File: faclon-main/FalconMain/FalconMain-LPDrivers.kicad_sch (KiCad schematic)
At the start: 41 parts, among them Q17 Q_NMOS_GSD, Q18 Q_NMOS_GSD, Q19 Q_PMOS_LFPAK, Q20 Q_NMOS_GSD, Q21 Q_PMOS_GSD, U4 BD9E104FJ-E2, U5 AL8843QSP-13, U6 NCP164ASN330T1G

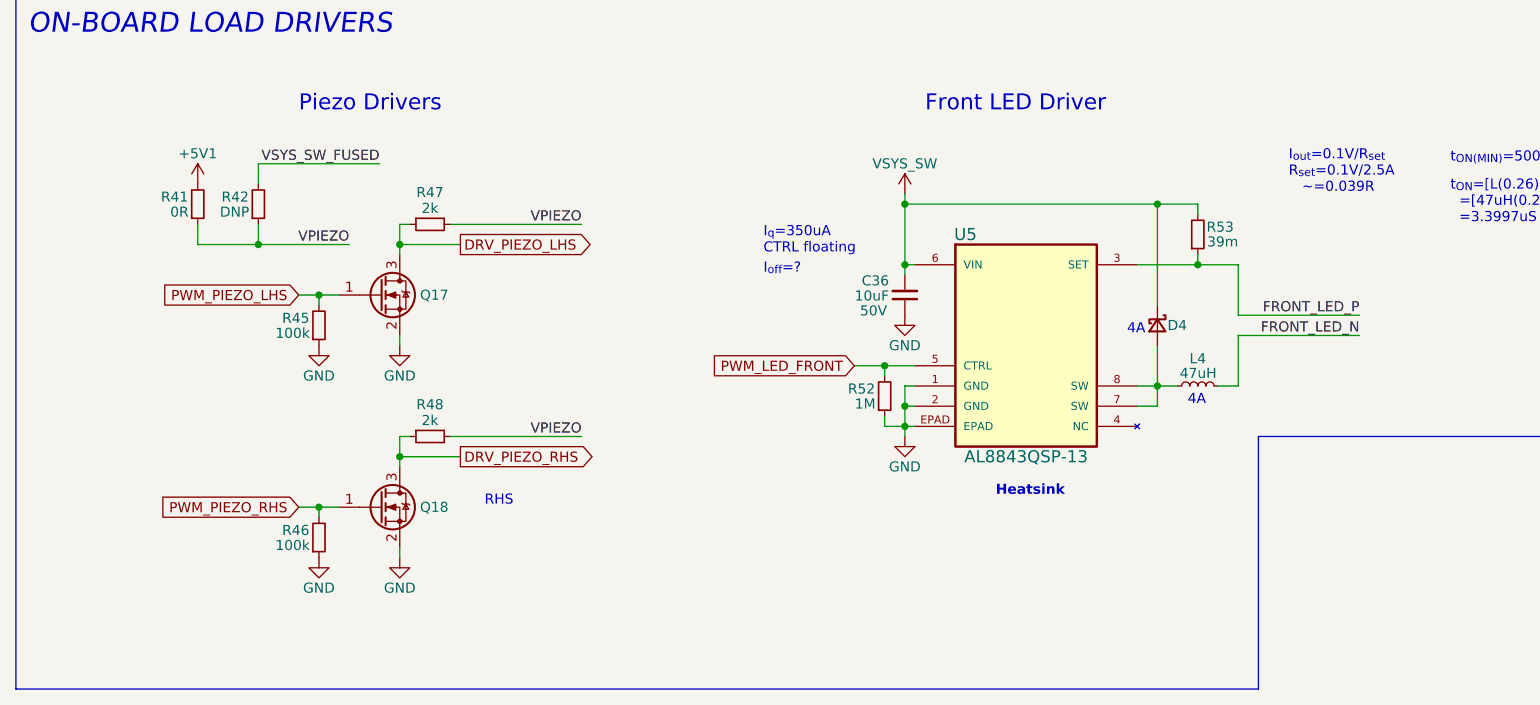
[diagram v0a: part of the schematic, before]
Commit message: Layour WIP
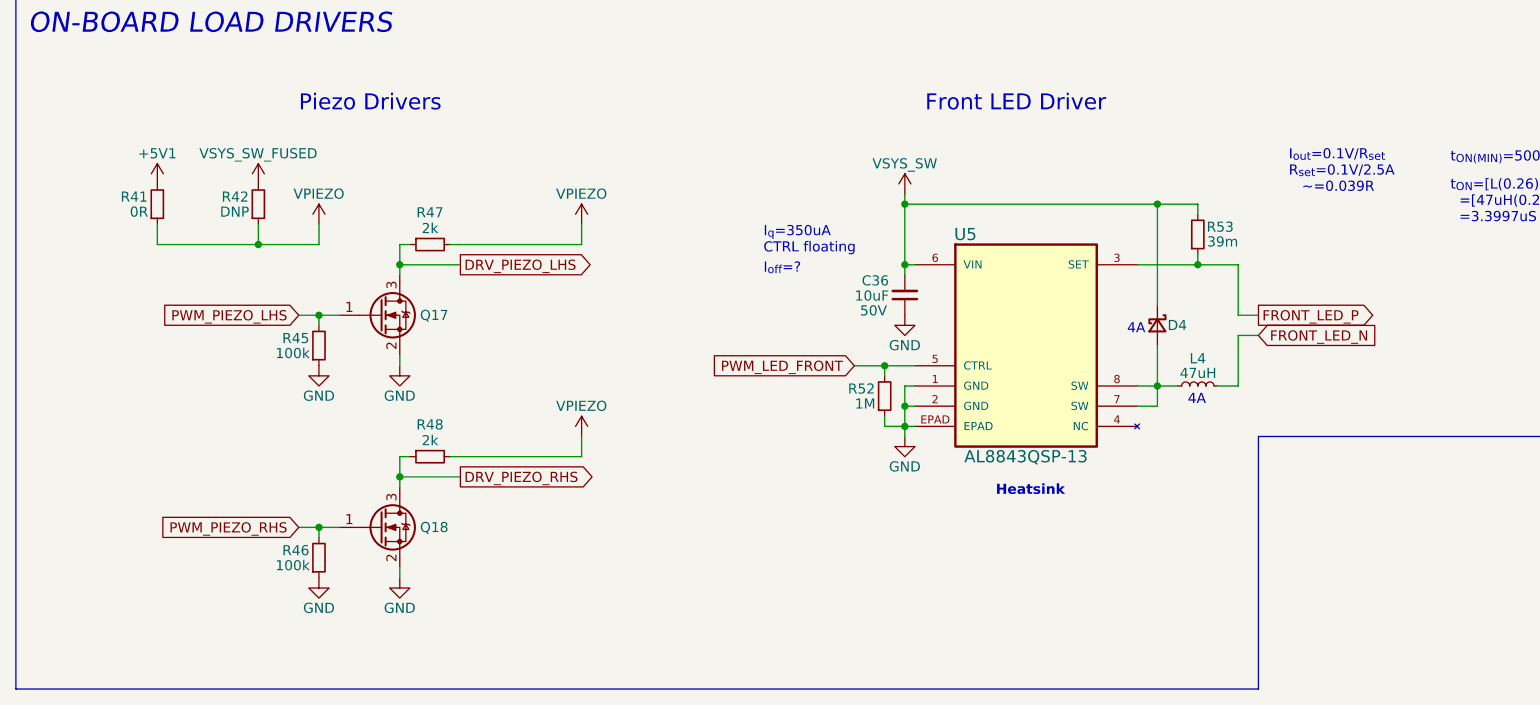
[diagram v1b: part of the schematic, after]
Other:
- note removed: "RHS"
- moved on the sheet: Q17, Q18, R41, R45, R46, R47, R48
